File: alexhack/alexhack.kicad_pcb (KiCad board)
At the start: 2 copper layers, 66.2 x 61.5 mm, 14 parts, among them J1 ultra, J2 battery, U1 ESP32_NODEMCU, U2 LM7805_TO220

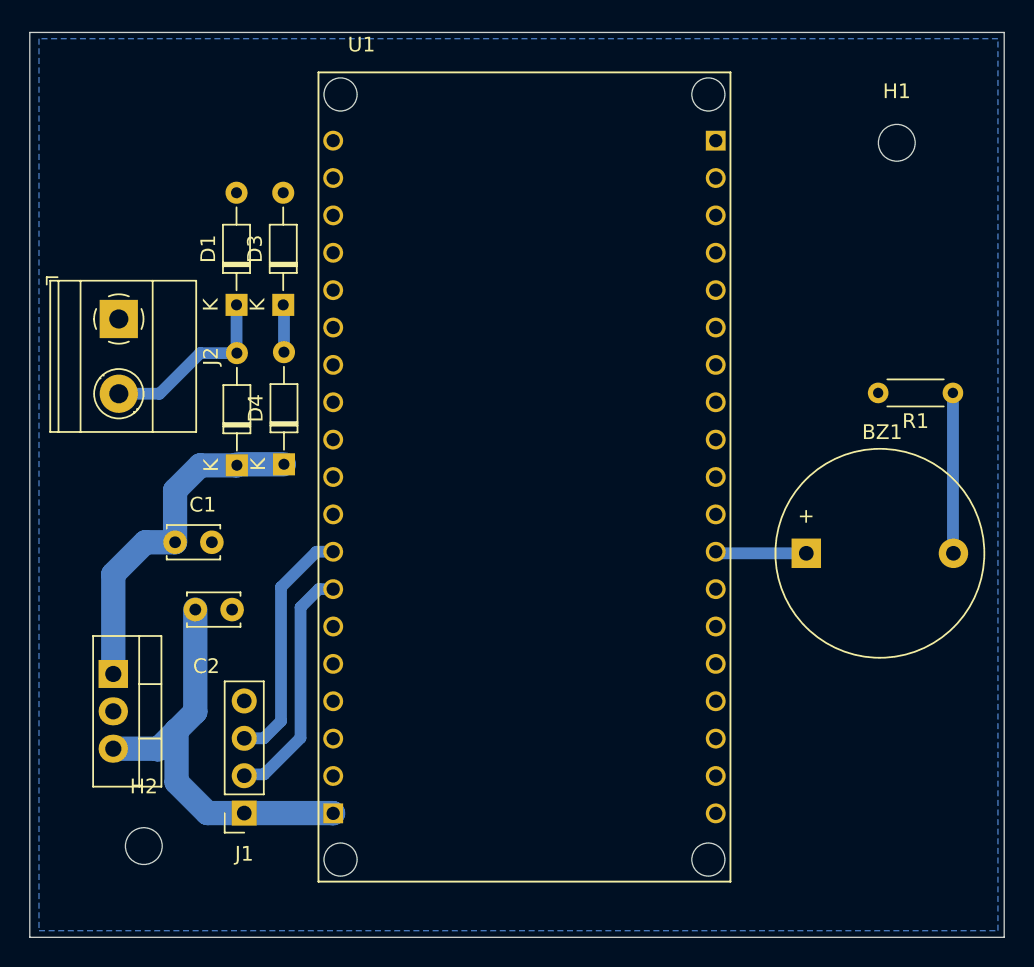
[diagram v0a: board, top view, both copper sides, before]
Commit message: Demo
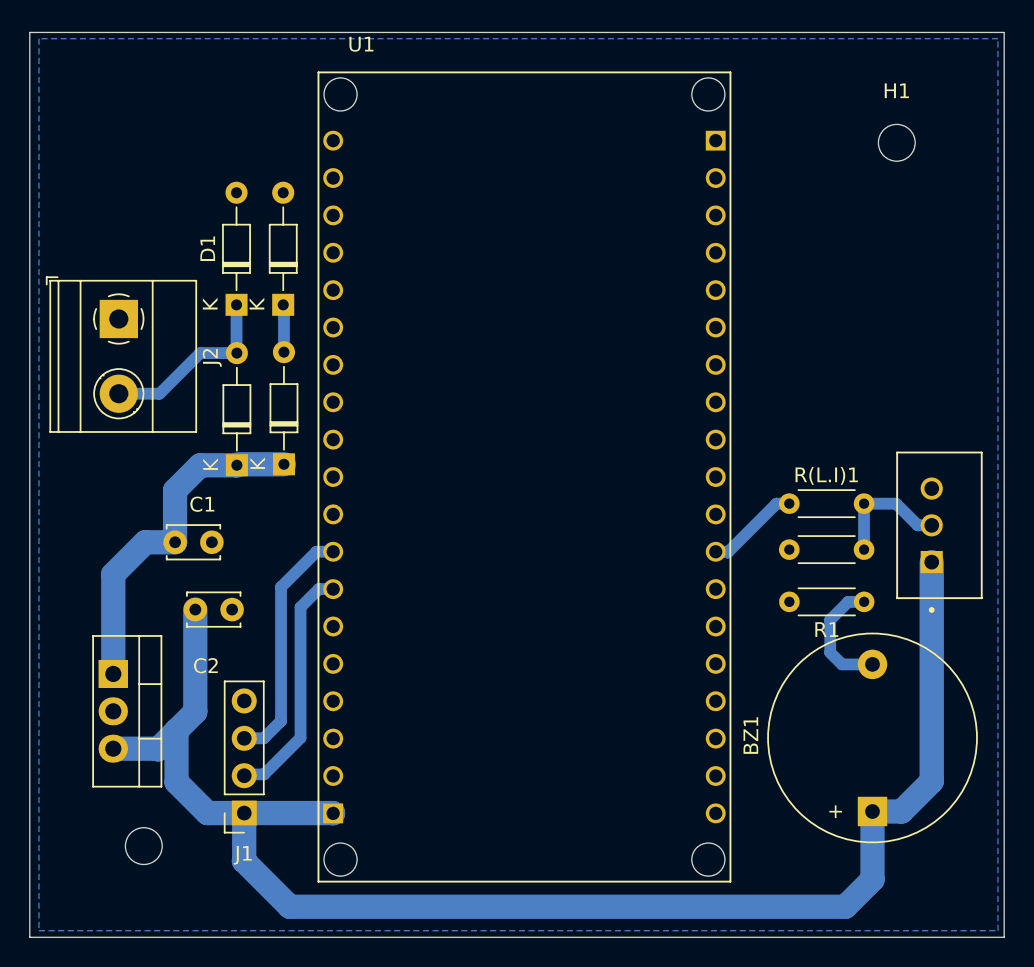
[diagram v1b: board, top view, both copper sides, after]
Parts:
- added Q1: NPN, B3B-XH-A_LF__SN_:JST_B3B-XH-A_LF__SN_, F.Cu at (168.2, 90.3)
- added R(L.I)1: 100, Resistor_THT:R_Axial_DIN0204_L3.6mm_D1.6mm_P5.08mm_Horizontal, F.Cu at (158.0, 88.9)
- added R(pd)1: 1 K, Resistor_THT:R_Axial_DIN0204_L3.6mm_D1.6mm_P5.08mm_Horizontal, F.Cu at (158.0, 92.0)
- moved BZ1 18.1 mm to (163.6, 109.8), turned to 90 degrees
- moved R1 15.4 mm to (163.1, 95.5)
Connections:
- BZ1 pad 1: Net-(BZ1-+) -> +5V
- U1 pad J4_12: Net-(BZ1-+) -> /15~
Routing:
- net +5V: track 28.6 -> 101.1 mm
- net Net-(Q1-B): track 0.00 -> 8.34 mm
- net /15~: track 0.00 -> 6.61 mm
- net Net-(BZ1-+): track 6.20 -> 0.00 mm
- net Net-(BZ1--): track 10.9 -> 8.24 mm
